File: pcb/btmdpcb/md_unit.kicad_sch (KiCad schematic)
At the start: 18 parts, among them SW1 SW_SPST, SW2 SW_Push, SW3 SW_SPST

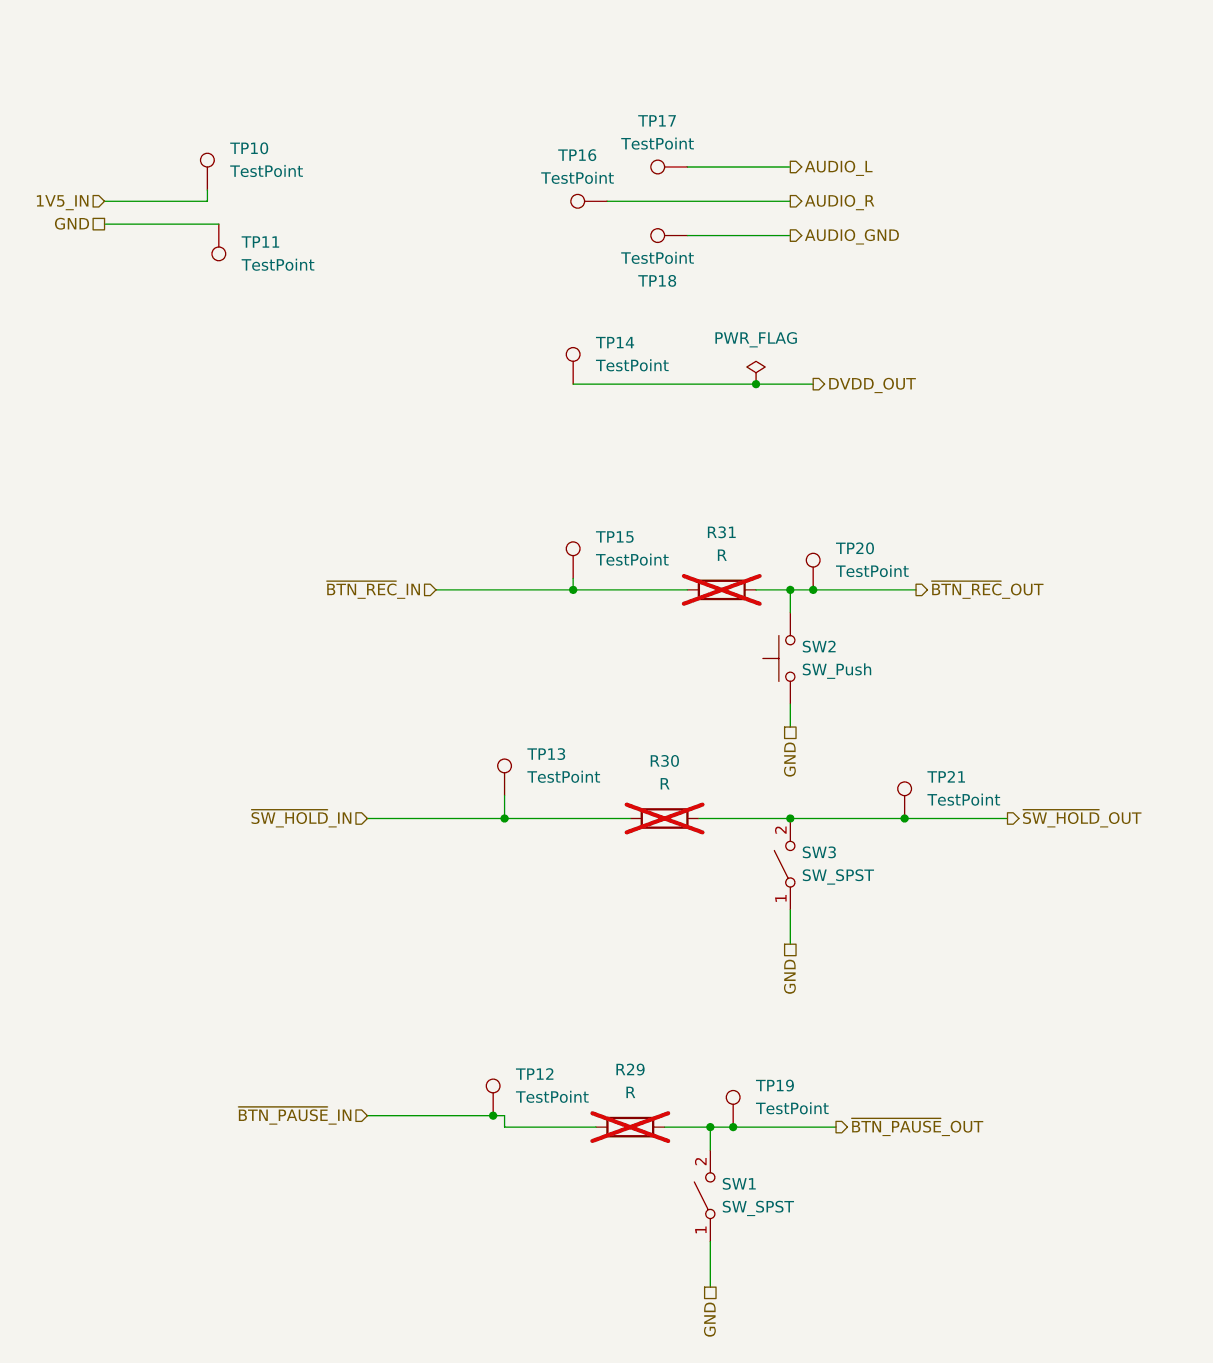
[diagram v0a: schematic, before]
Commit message: Layout PCB
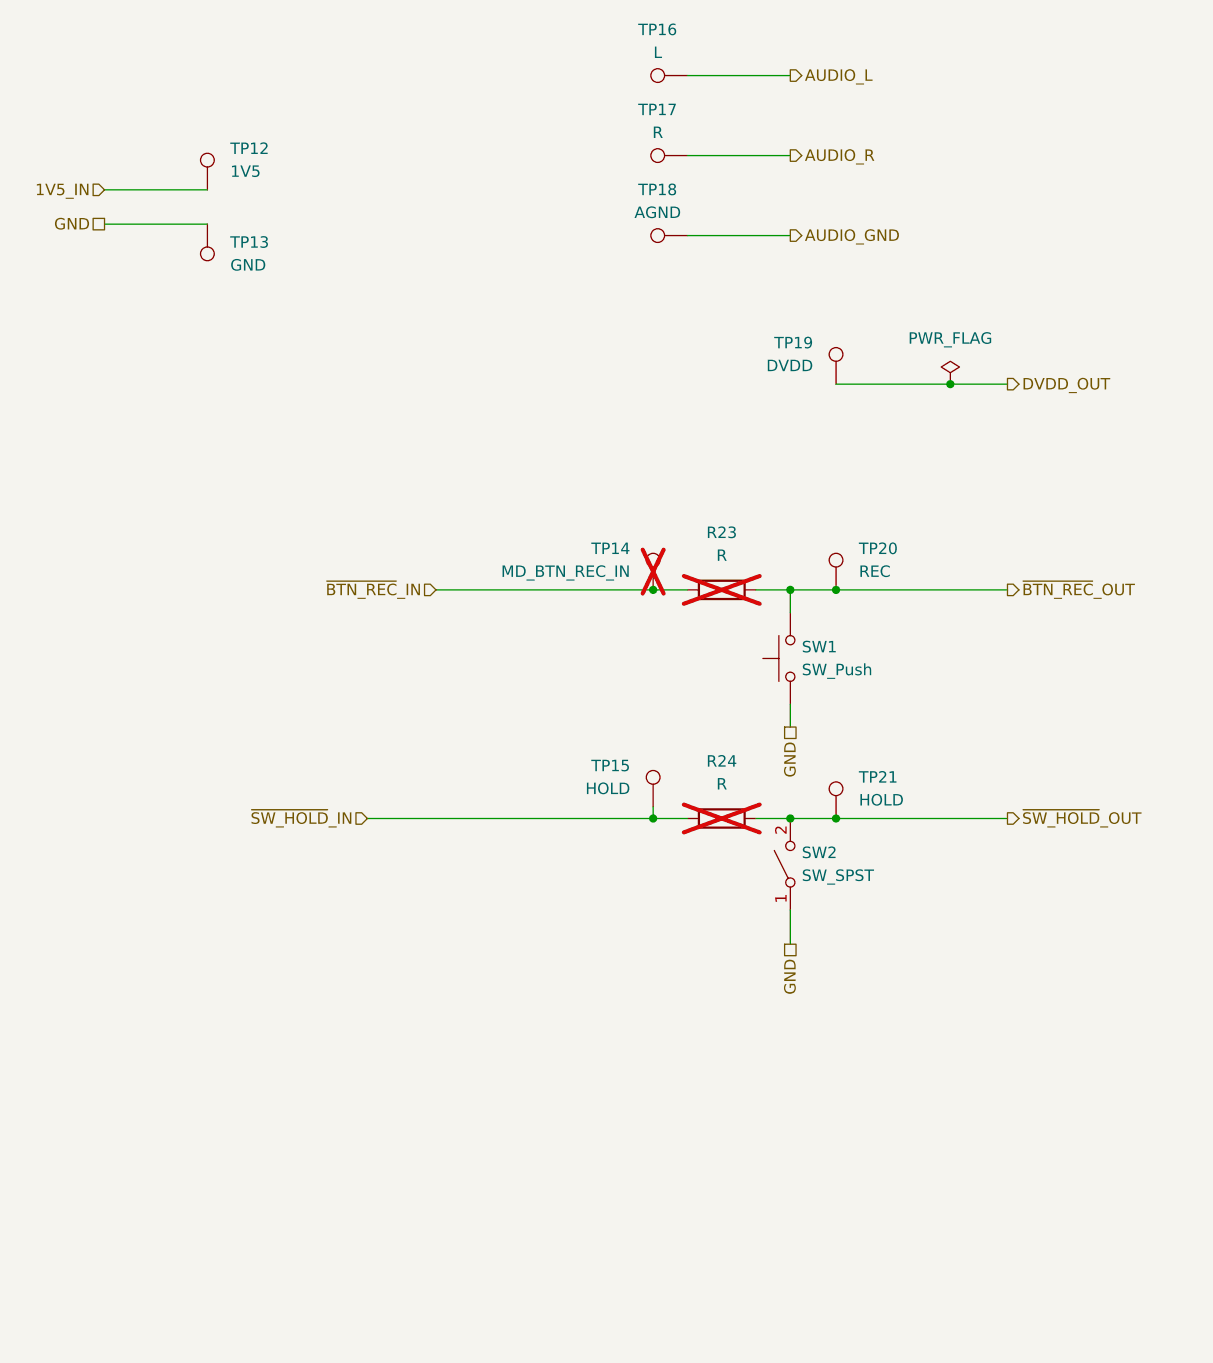
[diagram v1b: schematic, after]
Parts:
- removed R29: R, symbol Device:R
- removed SW1: SW_SPST, symbol Switch:SW_SPST
- removed TP12, TP19: TestPoint, TestPoint:TestPoint_Pad_D1.0mm, symbol Connector:TestPoint
- TP12: renamed from TP10; value TestPoint -> 1V5
- TP13: renamed from TP11; value TestPoint -> GND
- TP14: renamed from TP15; value TestPoint -> MD_BTN_REC_IN; now not fitted
- TP15: renamed from TP13; value TestPoint -> HOLD
- TP16: renamed from TP17; value TestPoint -> L
- TP17: renamed from TP16; value TestPoint -> R
- TP18: value TestPoint -> AGND
- TP19: renamed from TP14; value TestPoint -> DVDD
- TP20: value TestPoint -> REC
- TP21: value TestPoint -> HOLD
- renumbered R31 to R23, R30 to R24, SW2 to SW1, SW3 to SW2
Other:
- moved on the sheet: R24, TP13, TP15, TP16, TP17, TP19, TP20, TP21
